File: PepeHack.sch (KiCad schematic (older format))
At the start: 23 parts, among them J1 SWD, J2 Bat, Q1 AO3407, Q2 AO3407, SW70 SW_Push, SW71 SW_DPDT_x2, U1 E73-2G4M08S1C-52840, U2 TP4054, U3 XC6220B331MR, Y1 32.768kHz

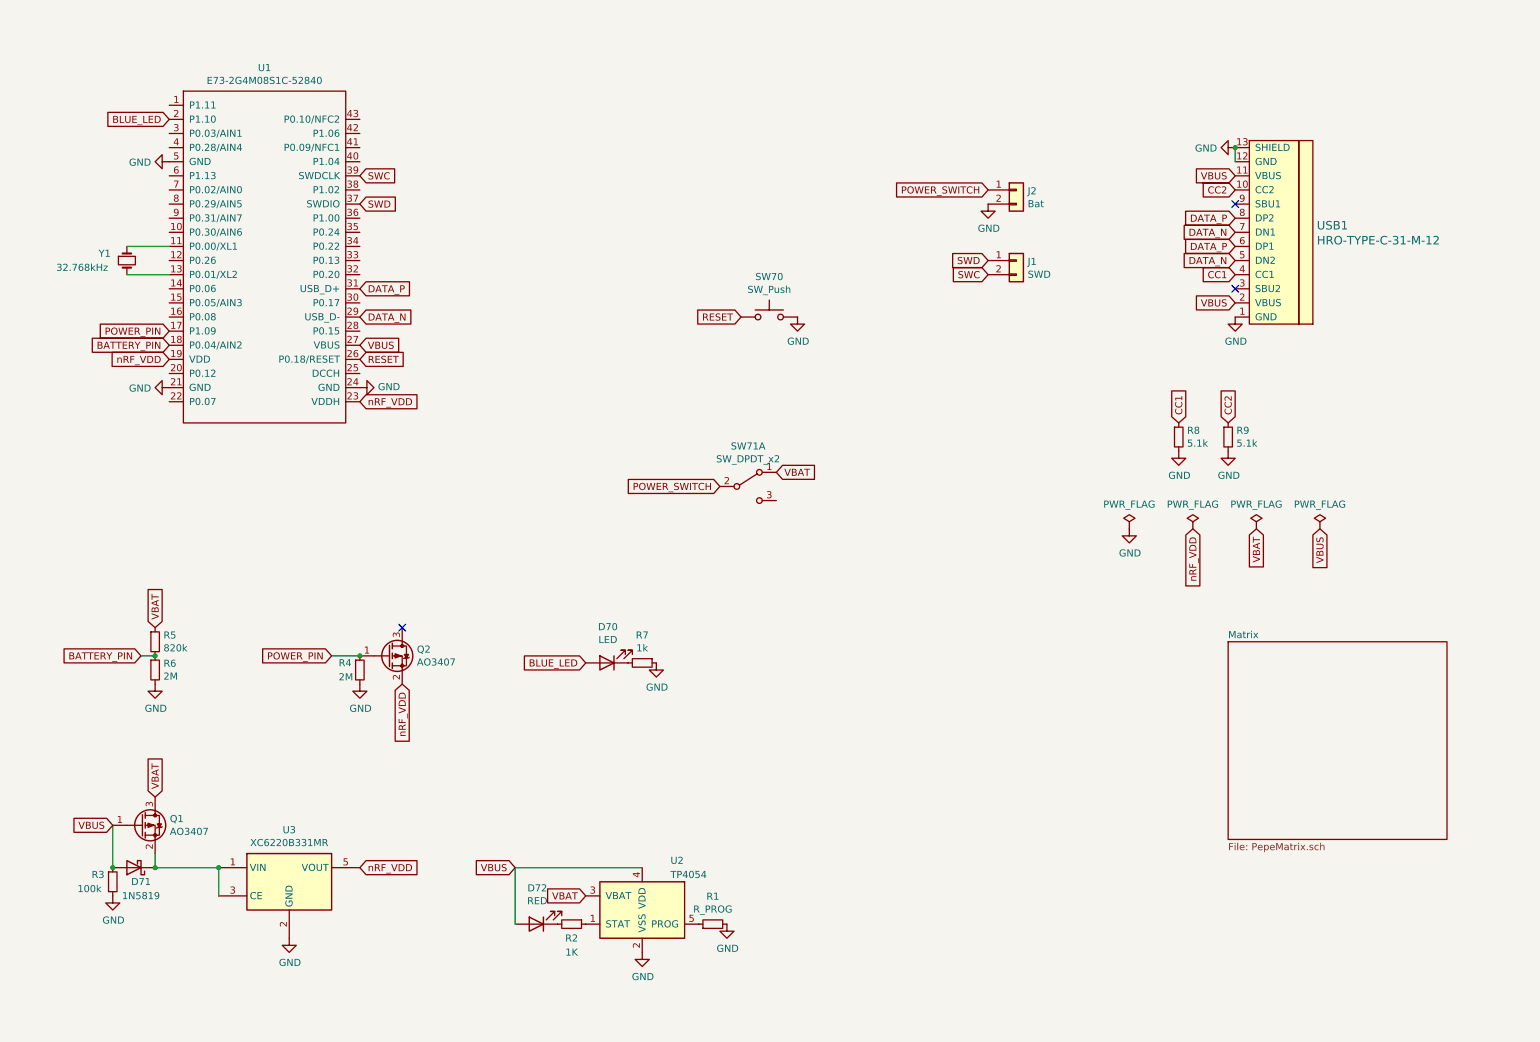
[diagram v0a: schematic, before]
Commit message: Trackball sensor
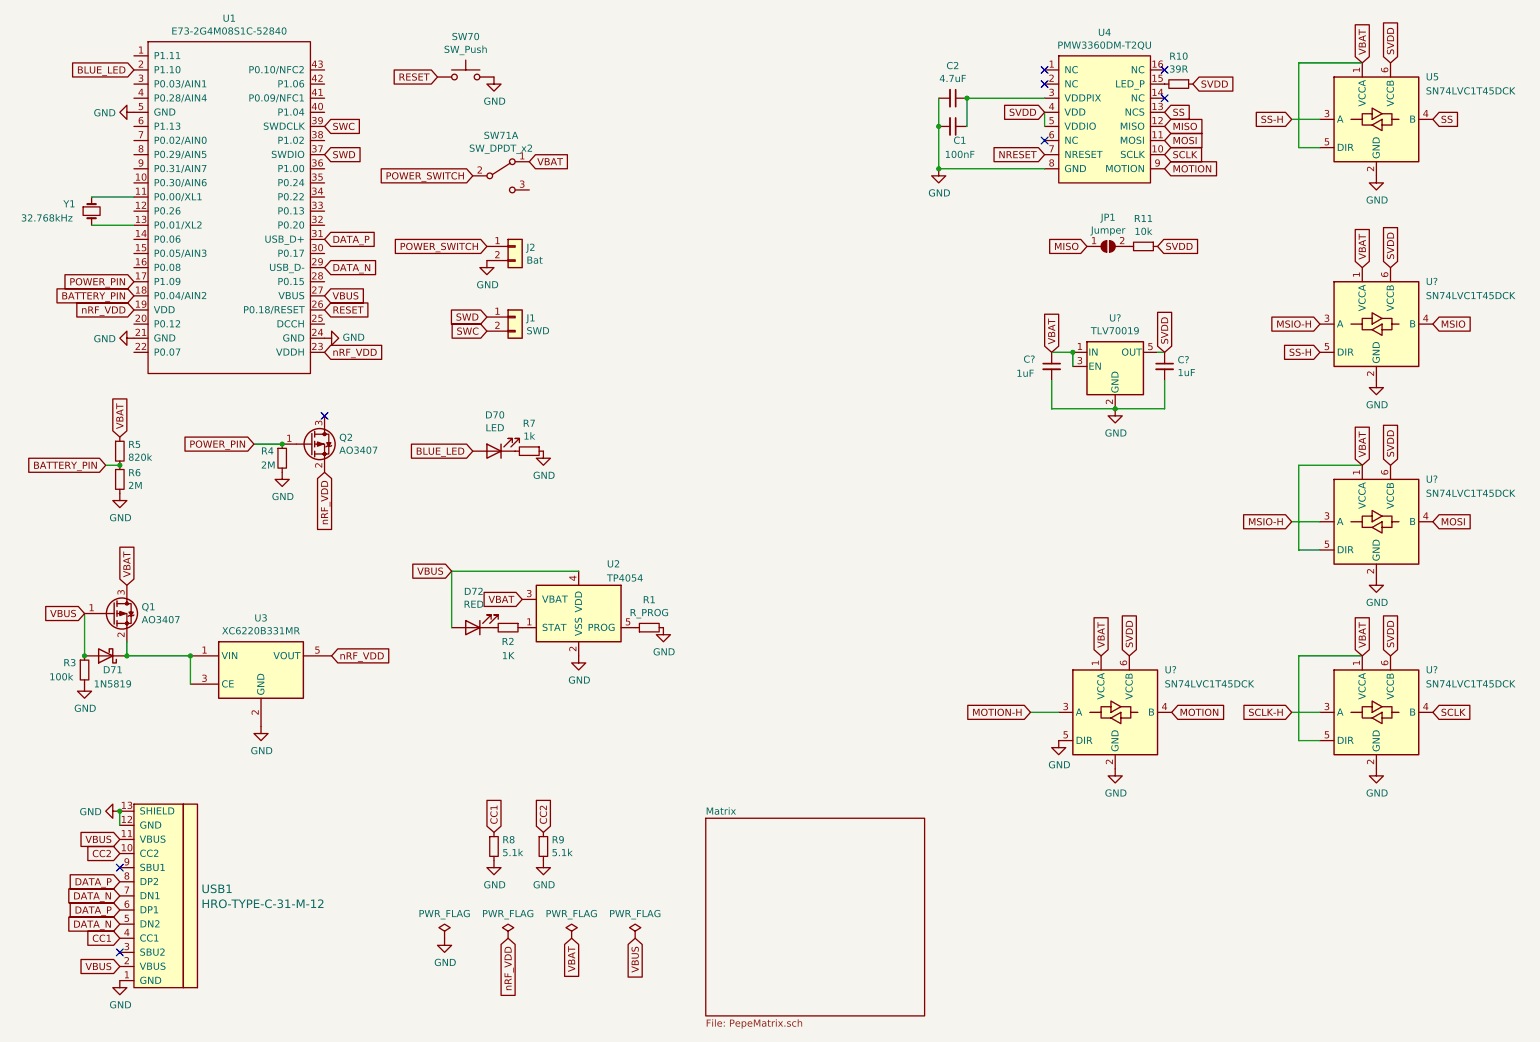
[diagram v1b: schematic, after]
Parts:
- added C1: 100nF, symbol Device:C_Small
- added C2: 4.7uF, symbol Device:C_Small
- added C? (x2): 1uF, symbol Device:C_Small
- added JP1: Jumper, symbol Jumper:SolderJumper_2_Open
- added R10: 39R, symbol Device:R_Small
- added R11: 10k, symbol Device:R_Small
- added U4: PMW3360DM-T2QU, symbol pmw3360dm-t2qu:PMW3360DM-T2QU
- added U5, U? (x4): SN74LVC1T45DCK, Package_TO_SOT_SMD:SOT-363_SC-70-6, symbol Logic_LevelTranslator:SN74LVC1T45DCK
- added U?: TLV70019, Package_TO_SOT_SMD:SOT-23-5, symbol Regulator_Linear:TLV70019_SOT23-5
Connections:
- net GND: now also C1.2, C2.2, C?.2, C?.2, U4.8 (GND), U5.2 (GND), U?.2 (GND), U?.2 (GND), U?.2 (GND), U?.2 (GND), U?.2 (GND), U?.5 (DIR)
- net VBAT: now also C?.1, U5.1 (VCCA), U5.5 (DIR), U?.1 (IN), U?.1 (VCCA), U?.1 (VCCA), U?.1 (VCCA), U?.1 (VCCA), U?.3 (EN), U?.5 (DIR), U?.5 (DIR)
- new net: R10.2, U4.15 (LED_P)
- new net: C1.1, C2.1, U4.3 (VDDPIX)
- new net: JP1.2 (B), R11.2
- new net MISO: JP1.1 (A), U4.12 (MISO)
- new net MOSI: U4.11 (MOSI), U?.4 (B)
- new net MOTION: U4.9 (MOTION), U?.4 (B)
- new net MOTION-H: U?.3 (A)
- new net MSIO: U?.4 (B)
- new net MSIO-H: U?.3 (A), U?.3 (A)
- new net NRESET: U4.7 (NRESET)
- new net SCLK: U4.10 (SCLK), U?.4 (B)
- new net SCLK-H: U?.3 (A)
- new net SS: U4.13 (NCS), U5.4 (B)
- new net SS-H: U5.3 (A), U?.5 (DIR)
- new net SVDD: C?.1, R10.1, R11.1, U4.4 (VDD), U4.5 (VDDIO), U5.6 (VCCB), U?.5 (OUT), U?.6 (VCCB), U?.6 (VCCB), U?.6 (VCCB), U?.6 (VCCB)
- no-connect marks 3 -> 8
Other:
- moved on the sheet: D70, D71, D72, J1, J2, Q1, Q2, R1, R2, R3, R4, R5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
